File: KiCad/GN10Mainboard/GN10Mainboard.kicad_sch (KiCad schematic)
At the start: 126 parts, among them J1 XT30PW-M, J10 USB_C_Receptacle_USB2.0, J11 Conn_01x04, J12 Conn_01x04, J13 Conn_01x06, J14 Conn_01x06, J2 Conn_01x04, J3 Conn_01x04, J4 Conn_01x04, J5 Conn_01x06, J6 Conn_01x04, J7 Conn_01x04, J8 Conn_01x04, J9 RJ45_Bel_SI-60062-F, SW1 SW_Push, U1 TPS54560DDA, U10 BNO086, U11 FT231XS, U2 3.3V, U4 STM32G474RETx, U5 MCP2562-E-SN, U6 MCP2562-E-SN, U7 MCP2562-E-SN, U8 W5500, Y1 24MHz, Y3 25M, Y6 32.768kHz, Y7 32.768kHz

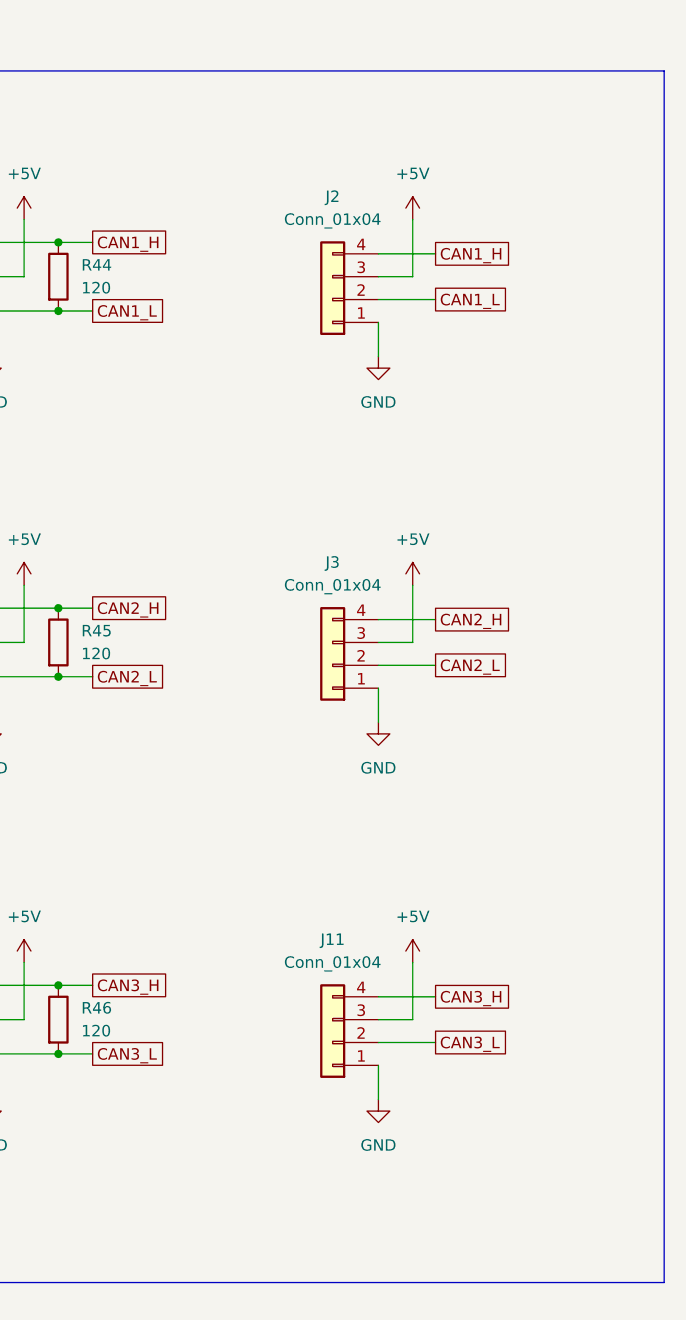
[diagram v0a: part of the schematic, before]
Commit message: update:PCB
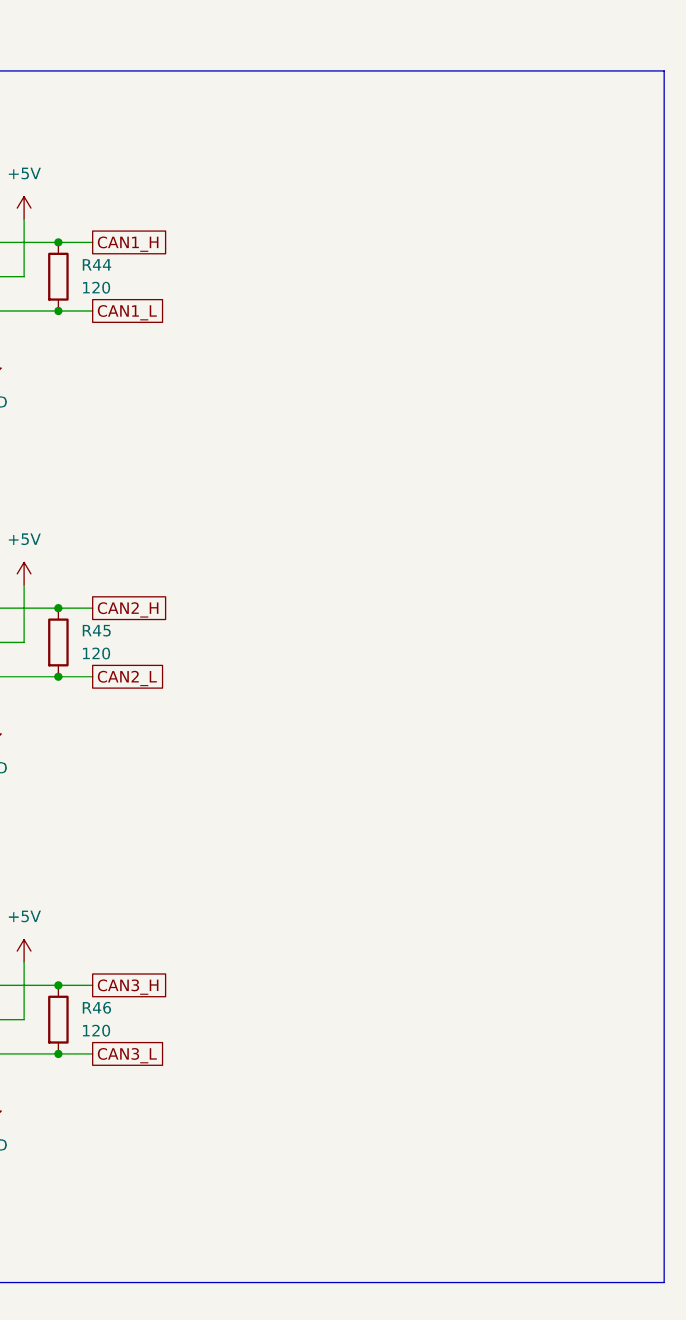
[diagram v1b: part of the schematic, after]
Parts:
- removed J11, J2, J3: Conn_01x04, Connector_JST:JST_XH_B4B-XH-A_1x04_P2.50mm_Vertical, symbol Connector_Generic:Conn_01x04
